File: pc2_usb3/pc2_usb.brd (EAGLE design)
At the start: 50 x 25 mm, 2 parts, among them K1 692141030100, K2 61400826021

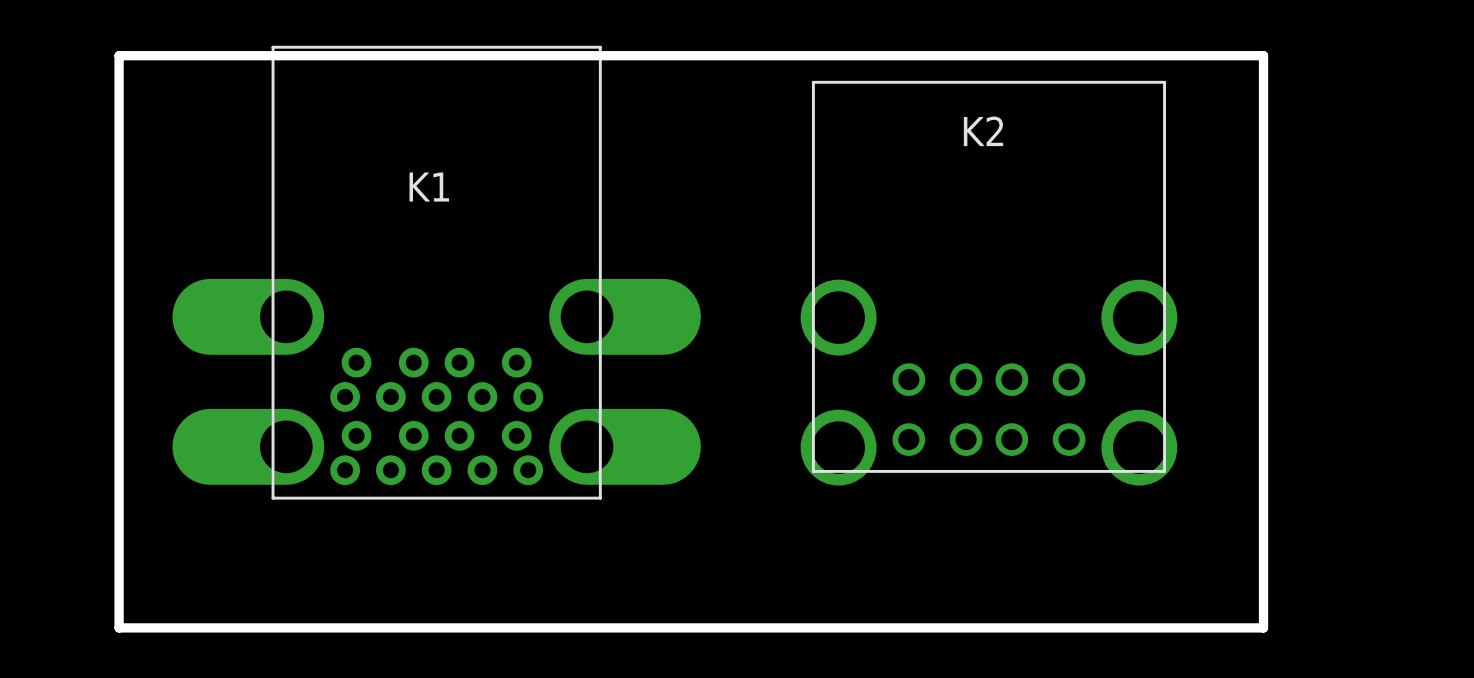
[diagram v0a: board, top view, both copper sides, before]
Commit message: .
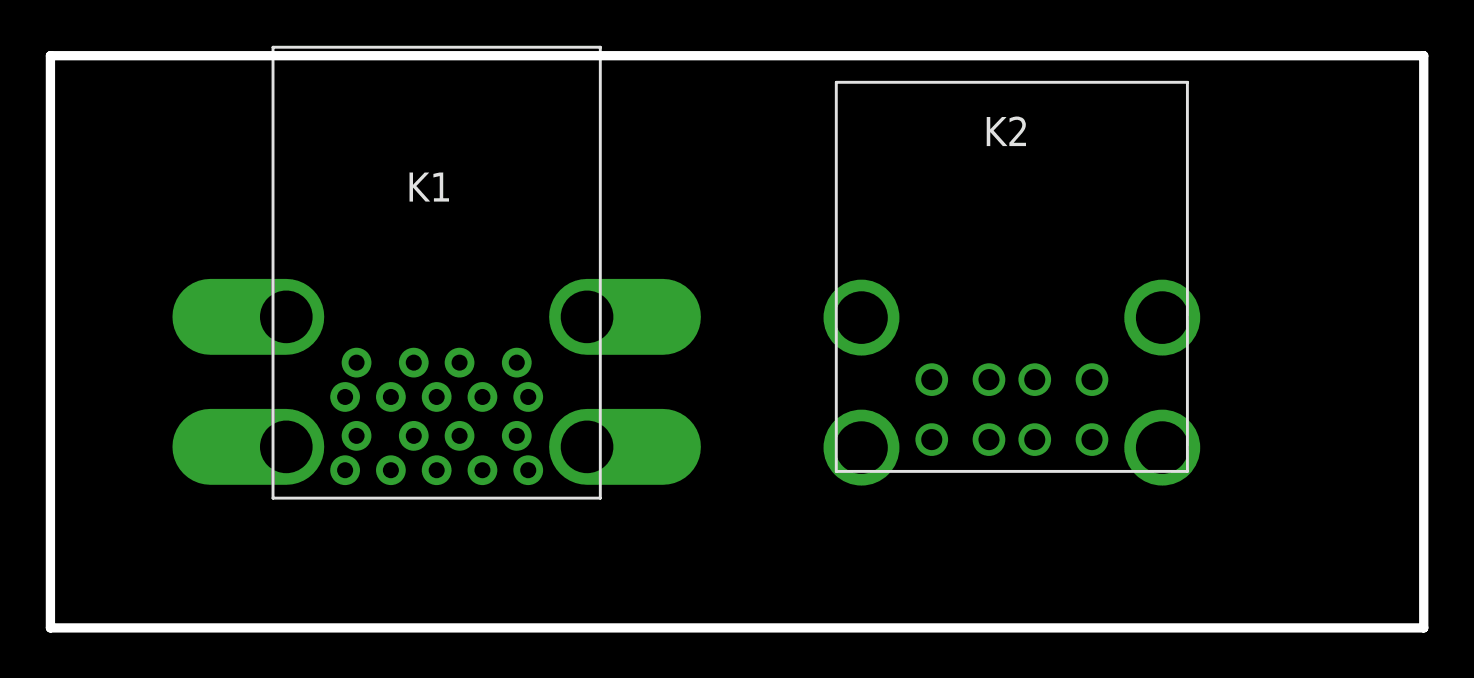
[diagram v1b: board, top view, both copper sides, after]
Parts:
- moved K2 1.00 mm to (41.0, 17.6)
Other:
- board size 50 x 25 mm -> 60 x 25 mm
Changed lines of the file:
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@@
 <board>
 <plain>
-<wire x1="2" y1="29" x2="52" y2="29" width="0.4064" layer="20"/>
-<wire x1="52" y1="29" x2="52" y2="4" width="0.4064" layer="20"/>
-<wire x1="52" y1="4" x2="2" y2="4" width="0.4064" layer="20"/>
-<wire x1="2" y1="4" x2="2" y2="29" width="0.4064" layer="20"/>
-<dimension x1="2" y1="33" x2="52" y2="33" x3="27" y3="42" textsize="1.778" layer="20" dtype="horizontal"/>
+<wire x1="-1" y1="29" x2="59" y2="29" width="0.4064" layer="20"/>
+<wire x1="59" y1="29" x2="59" y2="4" width="0.4064" layer="20"/>
+<wire x1="59" y1="4" x2="-1" y2="4" width="0.4064" layer="20"/>
+<wire x1="-1" y1="4" x2="-1" y2="29" width="0.4064" layer="20"/>
+<dimension x1="-1" y1="32" x2="59" y2="32" x3="29" y3="42" textsize="1.778" layer="20" dtype="horizontal"/>
 <dimension x1="-2" y1="29" x2="-2" y2="4" x3="-15" y3="16.5" textsize="1.778" layer="20" dtype="vertical"/>
+<dimension x1="49" y1="-8" x2="59" y2="-9" x3="54" y3="58" textsize="1.778" layer="20" dtype="horizontal"/>
 </plain>
 <attributes>
@@
 <attribute name="NAME" x="14.5325" y="22.6275" size="1.27" layer="25"/>
 </element>
-<element name="K2" library="Wurth_Elektronik_Electromechanic_Input-Output_Connectors_rev15c" package="61400826021" value="61400826021" x="40.005" y="17.5575" smashed="yes" rot="R180">
-<attribute name="NAME" x="38.753" y="25.051" size="1.27" layer="25"/>
-<attribute name="VALUE" x="34.943" y="19.1521" size="1.27" layer="27"/>
+<element name="K2" library="Wurth_Elektronik_Electromechanic_Input-Output_Connectors_rev15c" package="61400826021" value="61400826021" x="41.005" y="17.5575" smashed="yes" rot="R180">
+<attribute name="NAME" x="39.753" y="25.051" size="1.27" layer="25"/>
+<attribute name="VALUE" x="35.943" y="19.1521" size="1.27" layer="27"/>
 </element>
 </elements>
